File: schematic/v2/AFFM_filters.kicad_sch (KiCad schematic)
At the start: 22 parts, among them K1 DIPxx-1Axx-11x, K2 DIPxx-1Axx-11x, K3 DIPxx-1Axx-11x, K4 DIPxx-1Axx-11x

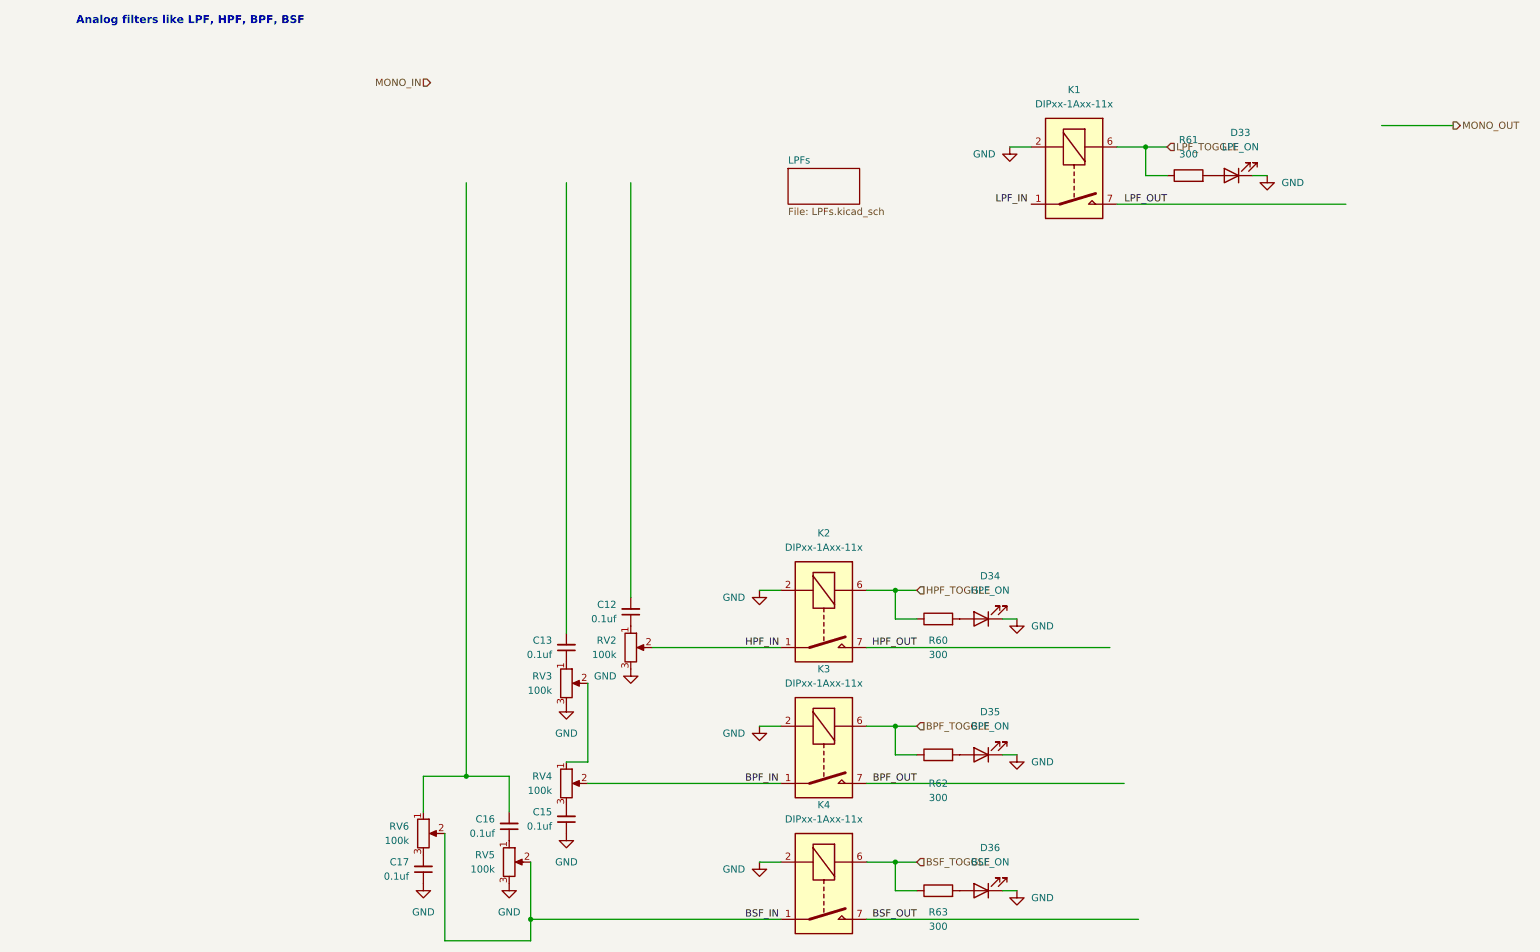
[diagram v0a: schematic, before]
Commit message: some progress on affm board
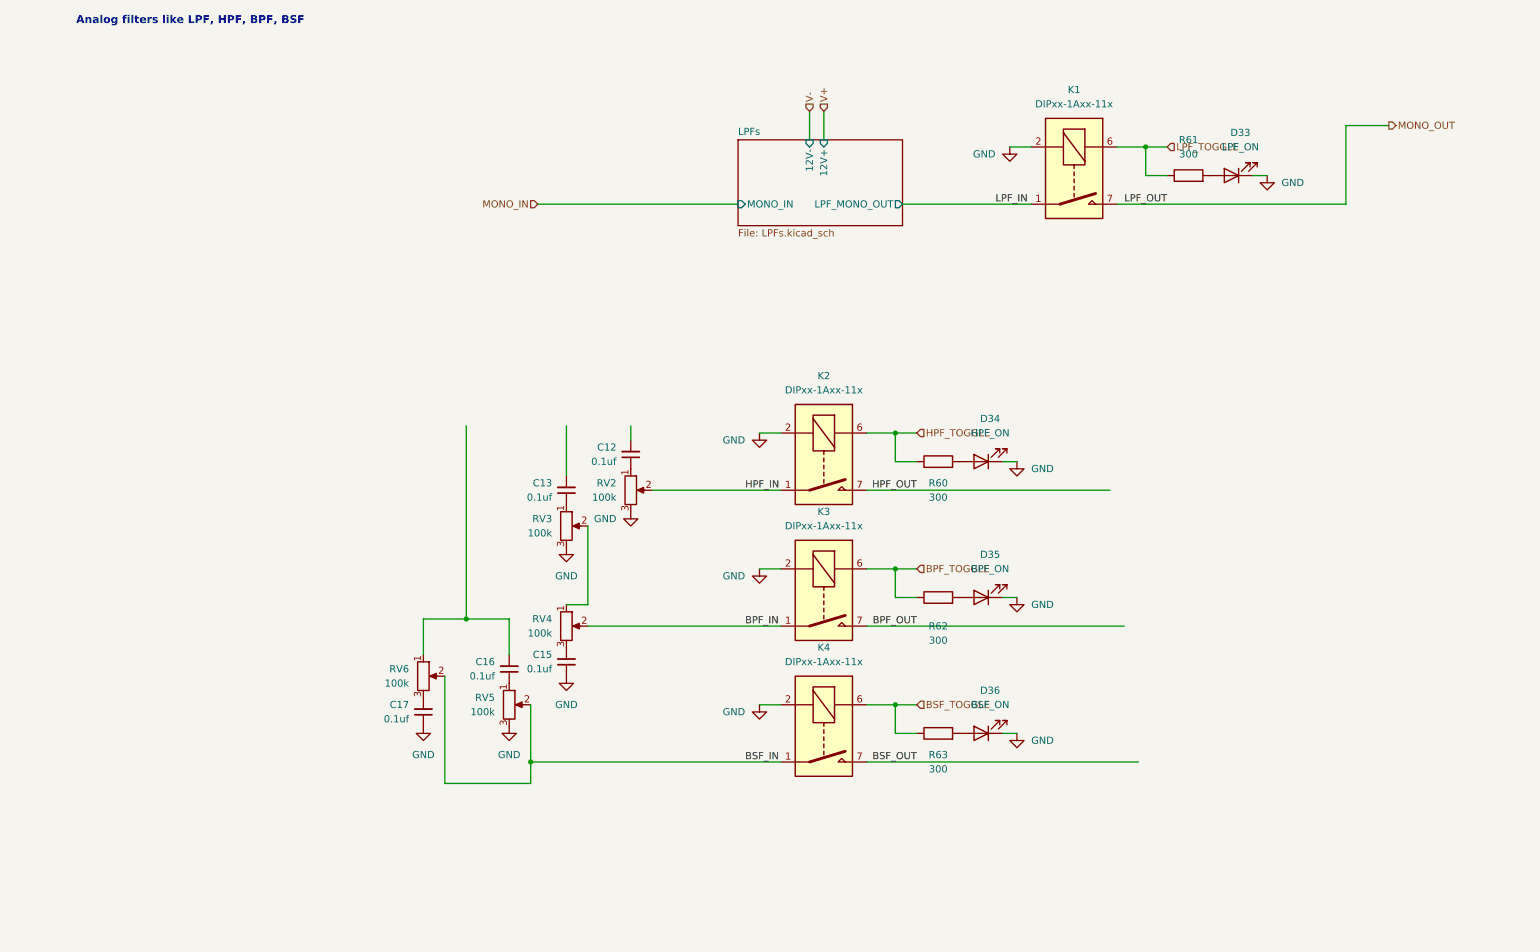
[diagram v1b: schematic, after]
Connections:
- net LPF_OUT is gone; now on net MONO_OUT: K1.7, K1.8
- net LPF_IN: now also K1.1, K1.14
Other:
- sheet LPFs ports: added 12V+, 12V-, LPF_MONO_OUT, MONO_IN; removed none
- moved on the sheet: C12, C13, C15, C16, C17, D34, D35, D36, K2, K3, K4, R60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
